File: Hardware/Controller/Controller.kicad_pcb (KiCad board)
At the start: 2 copper layers, 34.3 x 124.5 mm, 8 parts, among them J1 8P8C, U1 ESP32-WROOM-32D

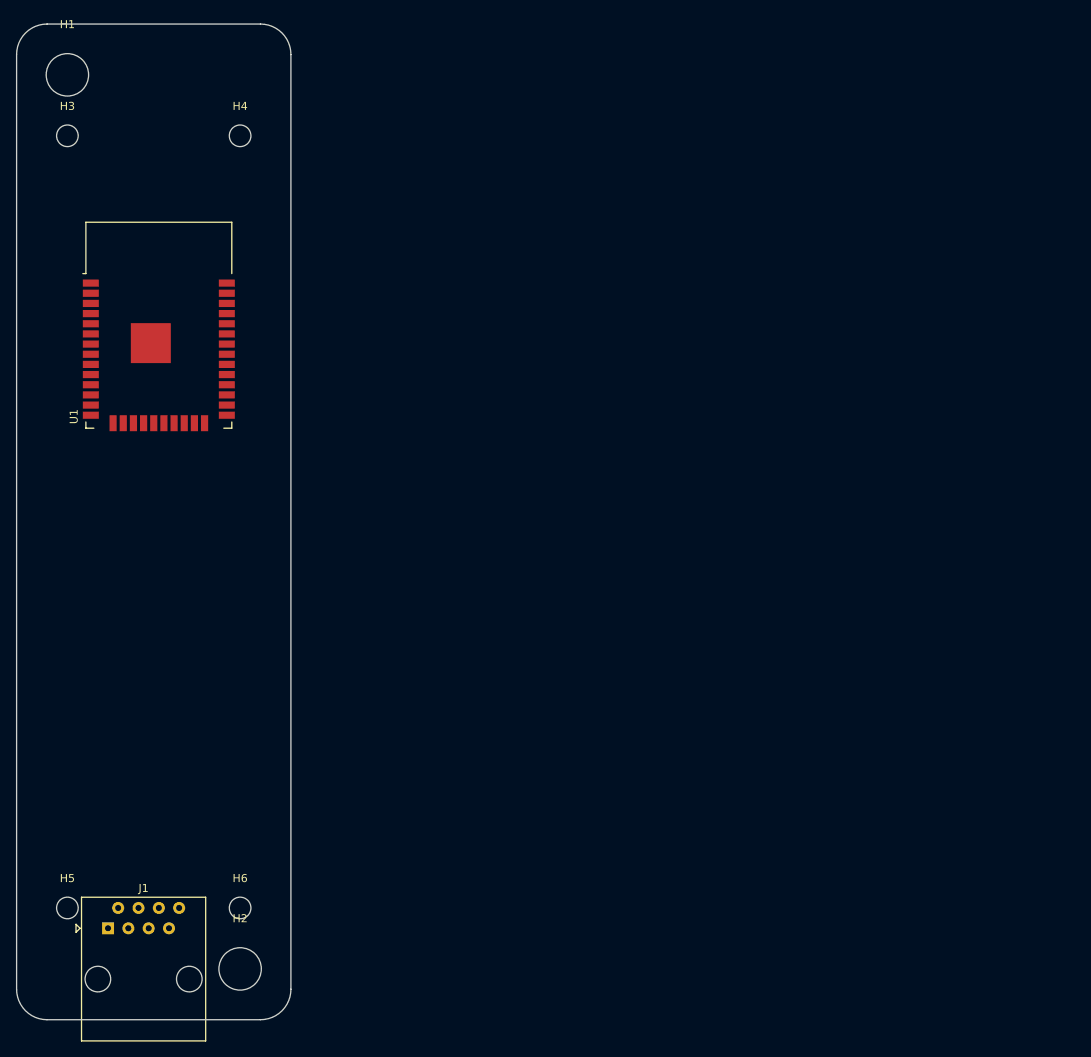
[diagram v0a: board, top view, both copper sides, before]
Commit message: Finished case-specific layout parts
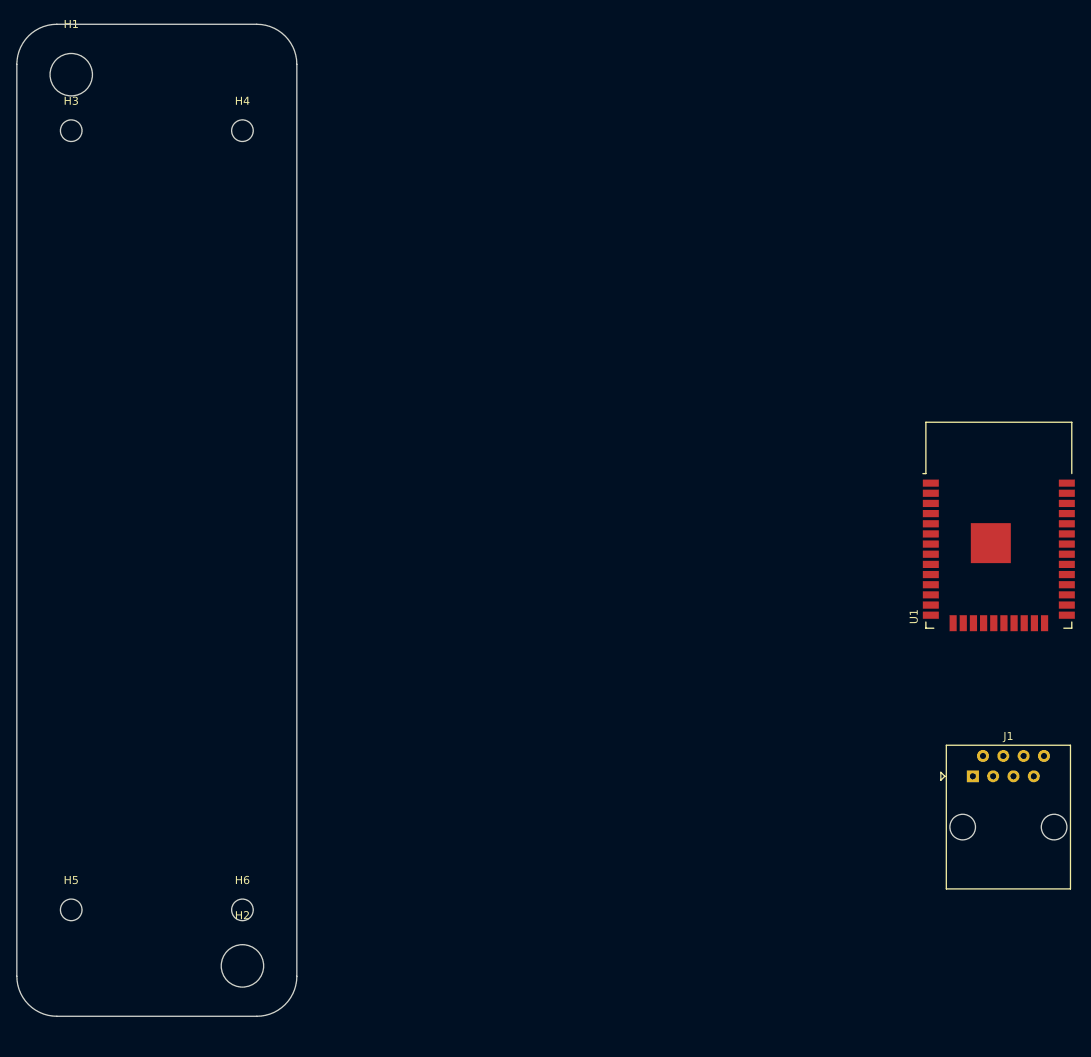
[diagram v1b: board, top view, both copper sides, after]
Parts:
- moved J1 109.8 mm to (133.5, 108.0)
- moved U1 107.9 mm to (136.8, 79.6)
- moved H3 0.80 mm to (20.8, 27.3)
- moved H4 0.70 mm to (42.2, 27.3)
- moved H5 0.54 mm to (20.8, 124.7)
- moved H1 0.48 mm to (20.8, 20.3)
- moved H2 0.48 mm to (42.2, 131.7)
- moved H6 0.38 mm to (42.2, 124.7)
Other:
- board size 34.3 x 124.5 mm -> 35 x 124 mm
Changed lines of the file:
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@@
   (general
     (thickness 1.6)
-    (drawings 10)
+    (drawings 9)
     (tracks 0)
     (zones 0)
@@
     (pad_to_mask_clearance 0.051)
     (solder_mask_min_width 0.25)
-    (aux_axis_origin 15.24 15.24)
+    (aux_axis_origin 13.97 13.97)
     (visible_elements 7FFFFFFF)
     (pcbplotparams
@@
   )
   (module MountingHole:MountingHole_5.3mm_M5 (layer F.Cu)
-    (at 20.32 20.32)
+    (at 20.8 20.3)
     (descr "Mounting Hole 5.3mm, no annular, M5")
     (tags "mounting hole 5.3mm no annular m5")
@@
   )
   (module MountingHole:MountingHole_5.3mm_M5 (layer F.Cu)
-    (at 41.91 132.08)
+    (at 42.2 131.7)
     (descr "Mounting Hole 5.3mm, no annular, M5")
     (tags "mounting hole 5.3mm no annular m5")
@@
   )
   (module RF_Module:ESP32-WROOM-32 (layer F.Cu)
-    (at 31.75 54.61)
+    (at 136.75 79.61)
     (descr "Single 2.4 GHz Wi-Fi and Bluetooth combo chip https://www.espressif.com/sites/default/files/documentation/esp32-wroom-32_datasheet_en.pdf")
     (tags "Single 2.4 GHz Wi-Fi and Bluetooth combo  chip")
@@
   )
   (module Connector_RJ:RJ45_Amphenol_54602-x08_Horizontal (layer F.Cu)
-    (at 25.4 127)
+    (at 133.5 108)
     (descr "8 Pol Shallow Latch Connector, Modjack, RJ45 (https://cdn.amphenol-icc.com/media/wysiwyg/files/drawing/c-bmj-0102.pdf)")
     (tags RJ45)
@@
   )
   (module MountingHole:MountingHole_2.7mm_M2.5 (layer F.Cu)
-    (at 20.32 27.94)
+    (at 20.8 27.3)
     (descr "Mounting Hole 2.7mm, no annular, M2.5")
     (tags "mounting hole 2.7mm no annular m2.5")
@@
   )
   (module MountingHole:MountingHole_2.7mm_M2.5 (layer F.Cu)
-    (at 41.91 27.94)
+    (at 42.2 27.3)
     (descr "Mounting Hole 2.7mm, no annular, M2.5")
     (tags "mounting hole 2.7mm no annular m2.5")
@@
   )
   (module MountingHole:MountingHole_2.7mm_M2.5 (layer F.Cu)
-    (at 20.32 124.46)
+    (at 20.8 124.7)
     (descr "Mounting Hole 2.7mm, no annular, M2.5")
     (tags "mounting hole 2.7mm no annular m2.5")
@@
   )
   (module MountingHole:MountingHole_2.7mm_M2.5 (layer F.Cu)
-    (at 41.91 124.46)
+    (at 42.2 124.7)
     (descr "Mounting Hole 2.7mm, no annular, M2.5")
     (tags "mounting hole 2.7mm no annular m2.5")
@@
     (pad 1 np_thru_hole circle (at 0 0) (size 2.7 2.7) (drill 2.7) (layers *.Cu *.Mask))
   )
-  (dimension 97.79 (width 0.3) (layer F.SilkS)
-    (gr_text "97,790 mm" (at 59.25 76.835 270) (layer F.SilkS)
-      (effects (font (size 1.5 1.5) (thickness 0.3)))
-    )
-    (feature1 (pts (xy 52.07 125.73) (xy 57.736421 125.73)))
-    (feature2 (pts (xy 52.07 27.94) (xy 57.736421 27.94)))
-    (crossbar (pts (xy 57.15 27.94) (xy 57.15 125.73)))
-    (arrow1a (pts (xy 57.15 125.73) (xy 56.563579 124.603496)))
-    (arrow1b (pts (xy 57.15 125.73) (xy 57.736421 124.603496)))
-    (arrow2a (pts (xy 57.15 27.94) (xy 56.563579 29.066504)))
-    (arrow2b (pts (xy 57.15 27.94) (xy 57.736421 29.066504)))
-  )
-  (target plus (at 15.24 15.24) (size 5) (width 0.15) (layer Edge.Cuts))
-  (gr_arc (start 17.78 134.62) (end 13.97 134.62) (angle -90) (layer Edge.Cuts) (width 0.15))
-  (gr_arc (start 44.45 134.62) (end 44.45 138.43) (angle -90) (layer Edge.Cuts) (width 0.15))
-  (gr_arc (start 17.78 17.78) (end 17.78 13.97) (angle -90) (layer Edge.Cuts) (width 0.15))
-  (gr_arc (start 44.45 17.78) (end 48.26 17.78) (angle -90) (layer Edge.Cuts) (width 0.15))
-  (gr_line (start 44.45 13.97) (end 17.78 13.97) (layer Edge.Cuts) (width 0.15))
-  (gr_line (start 48.26 134.62) (end 48.26 17.78) (layer Edge.Cuts) (width 0.15))
-  (gr_line (start 17.78 138.43) (end 44.45 138.43) (layer Edge.Cuts) (width 0.15))
-  (gr_line (start 13.97 17.78) (end 13.97 134.62) (layer Edge.Cuts) (width 0.15))
+  (gr_arc (start 19 133) (end 14 133) (angle -90) (layer Edge.Cuts) (width 0.15))
+  (gr_arc (start 44 133) (end 44 138) (angle -90) (layer Edge.Cuts) (width 0.15))
+  (gr_arc (start 44 19) (end 49 19) (angle -90) (layer Edge.Cuts) (width 0.15))
+  (gr_arc (start 19 19) (end 19 14) (angle -90) (layer Edge.Cuts) (width 0.15))
+  (gr_line (start 44 14) (end 19 14) (layer Edge.Cuts) (width 0.15))
+  (gr_line (start 49 133) (end 49 19) (layer Edge.Cuts) (width 0.15))
+  (gr_line (start 19 138) (end 44 138) (layer Edge.Cuts) (width 0.15))
+  (gr_line (start 14 19) (end 14 133) (layer Edge.Cuts) (width 0.15))
+  (target plus (at 31.5 76) (size 5) (width 0.15) (layer Edge.Cuts))
 )
